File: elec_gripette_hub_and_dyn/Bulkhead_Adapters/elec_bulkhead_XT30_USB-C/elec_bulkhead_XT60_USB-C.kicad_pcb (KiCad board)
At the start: 2 copper layers, 20 x 38.3 mm, 15 parts, among them J1 USB-C Rec. Vert., J2 JST EH 2, J3 XT60, J4 pico4, J5 Dynamixel-3, J9 Dynamixel-3

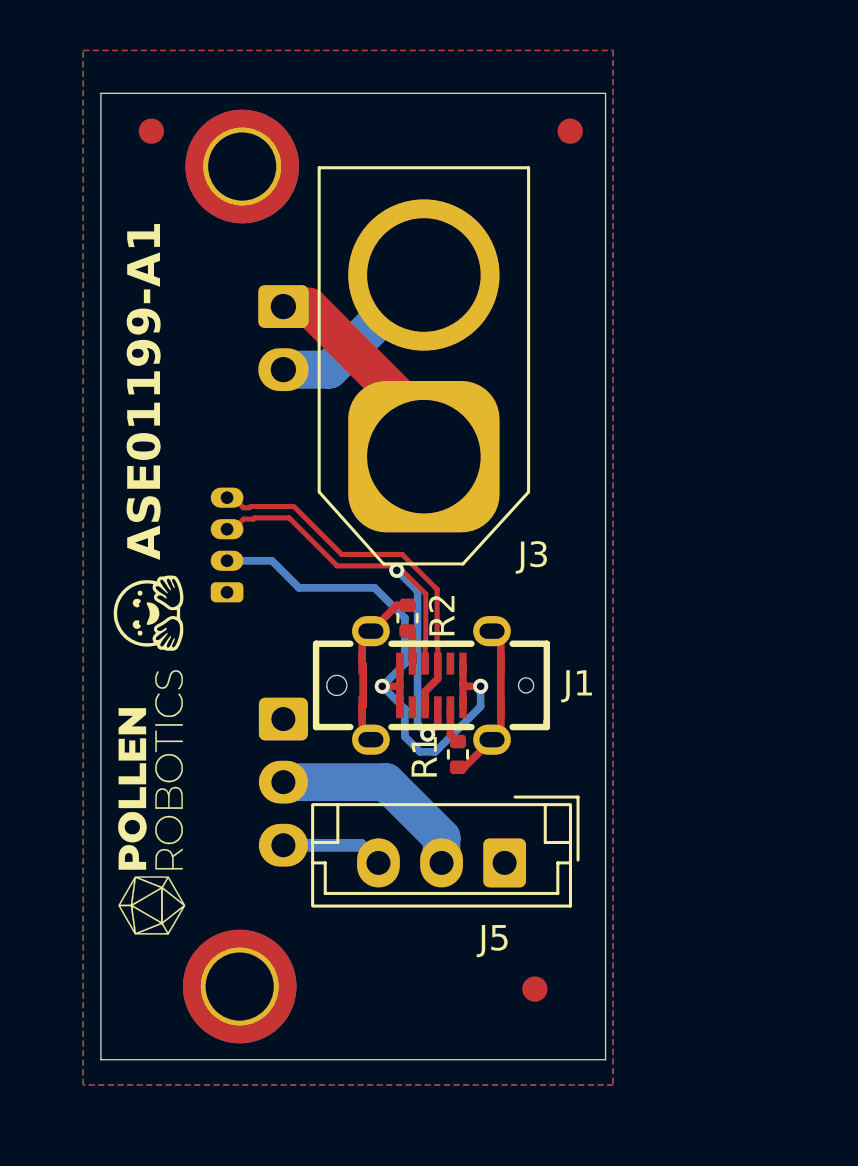
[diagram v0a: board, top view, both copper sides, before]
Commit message: [update] gripette + bulkhead -B1 in production @JLCPCB
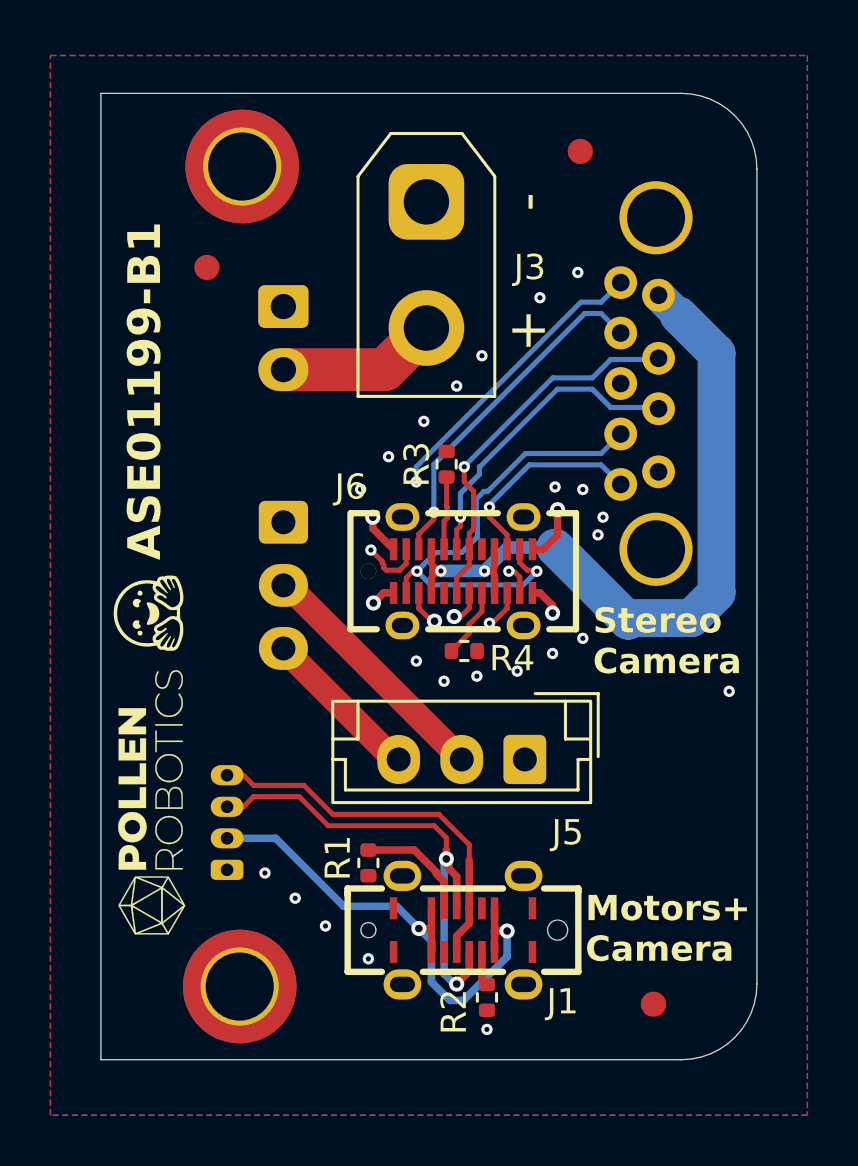
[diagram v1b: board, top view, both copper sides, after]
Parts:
- added J6: USB_C_Receptacle, LCSC_parts_lib:USB-C_TYPE-C-24PLT-H10.5-1, F.Cu at (93.4, 63.3)
- added J8: USB3_A, LCSC_parts_lib:USB-A-TH_MOLEX_484080003, B.Cu at (100.4, 55.8)
- added R3: 5k1, Resistor_SMD:R_0402_1005Metric, F.Cu at (92.8, 59.0)
- added R4: 5k1, Resistor_SMD:R_0402_1005Metric, F.Cu at (93.5, 66.4)
- J3: value XT60 -> XT30; footprint Connector_AMASS:AMASS_XT60-M_1x02_P7.20mm_Vertical -> Connector_AMASS:AMASS_XT30UPB-M_1x02_P5.0mm_Vertical
- moved R2 15.4 mm to (94.4, 80.2), turned to -90 degrees
- moved J4 11.0 mm to (84.1, 75.1)
- moved J3 10.1 mm to (92.0, 48.6), turned to -90 degrees
- moved J1 9.78 mm to (93.4, 77.5), turned to 0 degrees
- moved J9 7.80 mm to (86.3, 61.3)
- moved FID1 5.83 mm to (83.3, 51.2)
- moved R1 5.58 mm to (89.7, 74.8)
- moved FID3 4.74 mm to (101.0, 80.4)
- moved J5 4.18 mm to (95.9, 70.7)
- moved FID2 0.89 mm to (98.1, 46.6)
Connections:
- net VBUS renamed Net-(J4-Pin_2)
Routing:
- net Net-(J8-VBUS): track 0.00 -> 34.4 mm, vias 0 -> 2
- net /SSTx+: track 0.00 -> 25.7 mm, vias 0 -> 3
- net /SSTx-: track 0.00 -> 20.7 mm, vias 0 -> 2
- net /SSRx+: track 0.00 -> 19.0 mm, vias 0 -> 2
- net /D+: track 0.00 -> 17.7 mm, vias 0 -> 2
- net /SSRx-: track 0.00 -> 16.3 mm, vias 0 -> 2
- net GND: track 21.7 -> 6.12 mm, vias 0 -> 27
- net /D-: track 0.00 -> 14.9 mm, vias 0 -> 1
- net Net-(J1-CC1): track 1.48 -> 4.62 mm
- net Net-(J6-CC1): track 0.00 -> 2.92 mm
- net Net-(J6-CC2): track 0.00 -> 2.80 mm
- net Net-(J5-Pin_3): track 4.06 -> 6.39 mm
- net Net-(J4-Pin_2): track 23.1 -> 20.9 mm
- net Net-(J5-Pin_2): track 8.18 -> 9.93 mm
- net /DM+: track 20.3 -> 19.2 mm
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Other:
- board size 20 x 38.3 mm -> 26 x 38.3 mm
- copper layers 2 -> 4
- board text added: "1,6 mm PCB thickness 35 um (1 oz) copper"
- board text added: "ASE01199-B1"
- board text added: "Motors+ Camera"
- board text added: "Stereo Camera"
- board text removed: "1 mm PCB thickness 35 um (1 oz) copper"
- board text removed: "ASE01199-A1"
